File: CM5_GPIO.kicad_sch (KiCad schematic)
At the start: 26 parts, among them J10 JST_SHBM04B-SRSS-TB, J11 THD-20-R, J12 THD-02-R, J13 Micro_SD_Card_Det, J8 Conn_02x07_Odd_Even, J9 Conn_01x03, SW1 Right angle Tact button, U3 74LVC1G07SE-7, U4 TPD4EUSB30, U5 TPD4EUSB30, U6 RT9742GGJ5, U7 MagJack-A70-112-331N126

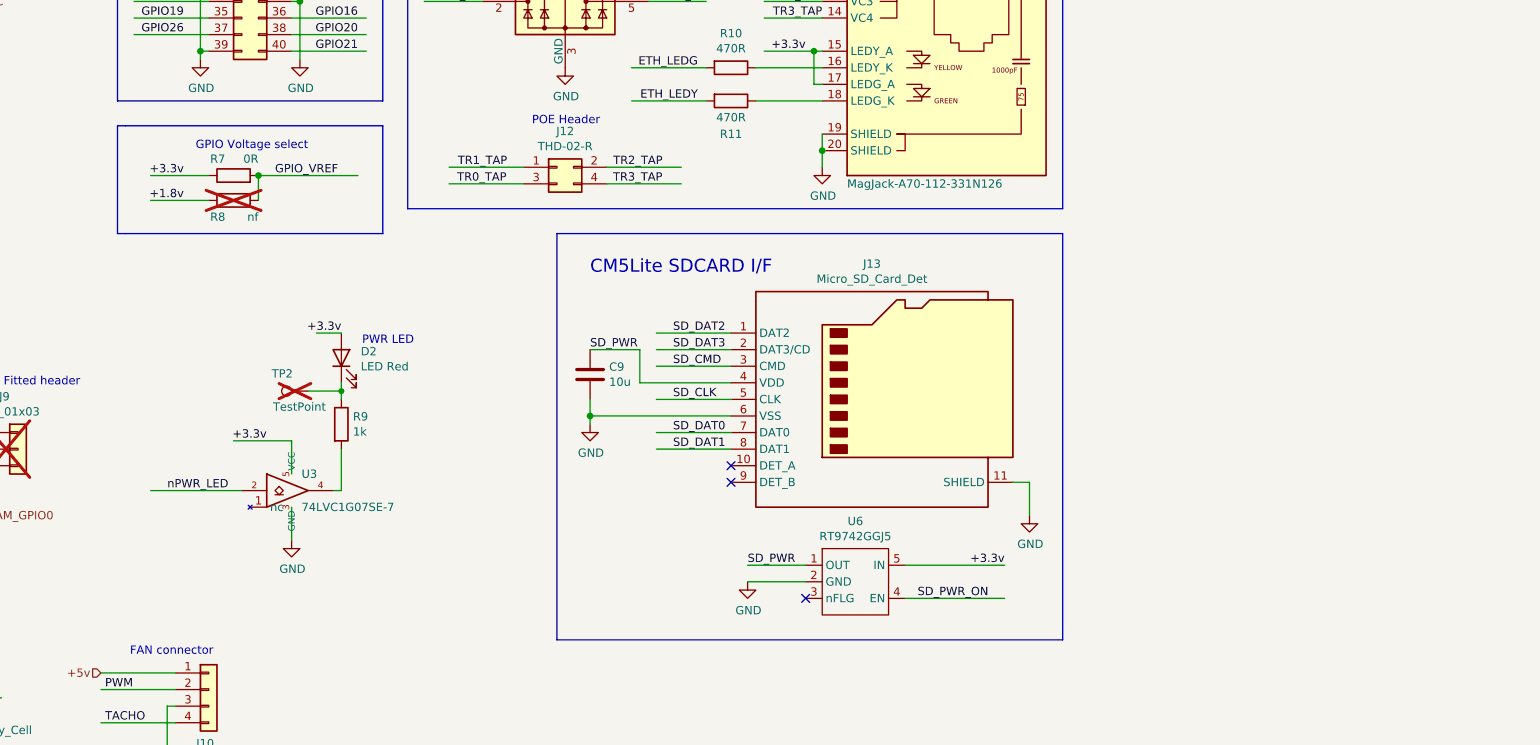
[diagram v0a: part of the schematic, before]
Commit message: complete schematic
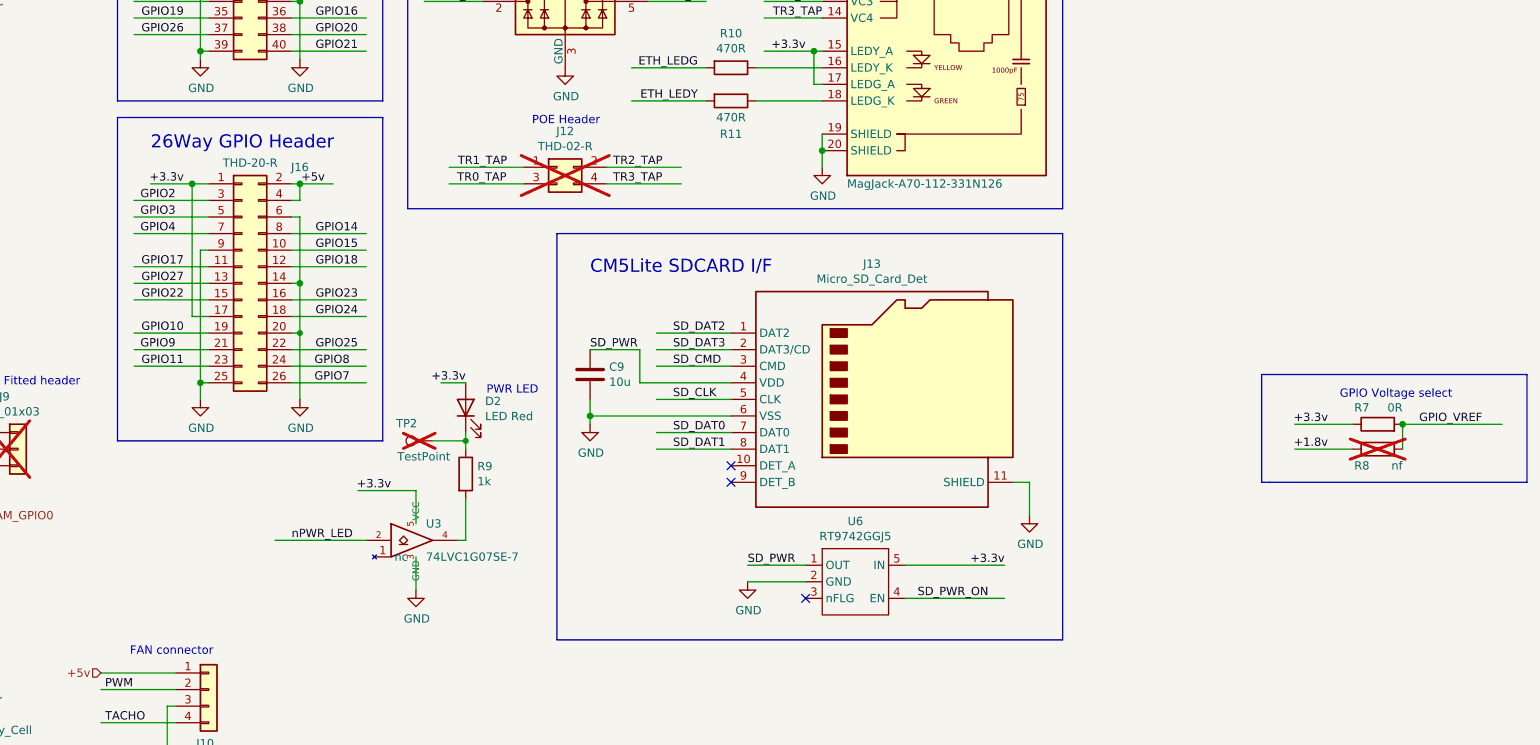
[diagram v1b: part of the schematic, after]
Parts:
- added J16: THD-20-R, Connector_IDC:IDC-Header_2x13_P2.54mm_Vertical, symbol Connector_Generic:Conn_02x20_Odd_Even
- BT1: digikey (none) -> 36-3034-ND
- C10: footprint Capacitor_SMD:C_0402_1005Metric -> Capacitor_SMD:C_0805_2012Metric_Pad1.18x1.45mm_HandSolder; digikey (none) -> 1276-1003-1-ND
- C9: footprint Capacitor_SMD:C_0805_2012Metric -> Capacitor_SMD:C_0805_2012Metric_Pad1.18x1.45mm_HandSolder; digikey (none) -> 1276-1096-1-ND
- D1: digikey (none) -> LTST-S270KGKT
- D2: digikey (none) -> LTST-S270KRKT
- J12: now not fitted
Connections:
- net +3.3v: now also J16.1 (Pin_1), J16.17 (Pin_17)
- net +5v: now also J16.2 (Pin_2), J16.4 (Pin_4)
- net GND: now also J16.14 (Pin_14), J16.20 (Pin_20), J16.25 (Pin_25), J16.6 (Pin_6), J16.9 (Pin_9)
- net GPIO10: now also J16.19 (Pin_19)
- net GPIO11: now also J16.23 (Pin_23)
- net GPIO14: now also J16.8 (Pin_8)
- net GPIO15: now also J16.10 (Pin_10)
- net GPIO17: now also J16.11 (Pin_11)
- net GPIO18: now also J16.12 (Pin_12)
- net GPIO2: now also J16.3 (Pin_3)
- net GPIO22: now also J16.15 (Pin_15)
- net GPIO23: now also J16.16 (Pin_16)
- net GPIO24: now also J16.18 (Pin_18)
- net GPIO25: now also J16.22 (Pin_22)
- net GPIO27: now also J16.13 (Pin_13)
- net GPIO3: now also J16.5 (Pin_5)
- net GPIO4: now also J16.7 (Pin_7)
- net GPIO7: now also J16.26 (Pin_26)
- net GPIO8: now also J16.24 (Pin_24)
- net GPIO9: now also J16.21 (Pin_21)
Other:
- note added: "26Way GPIO Header"
- moved on the sheet: D2, R7, R8, R9, TP2, U3
